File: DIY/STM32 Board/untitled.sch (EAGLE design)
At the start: 13 parts, among them IC2 REG1117, Q1 16 MHz, U1 STM32103RBT6

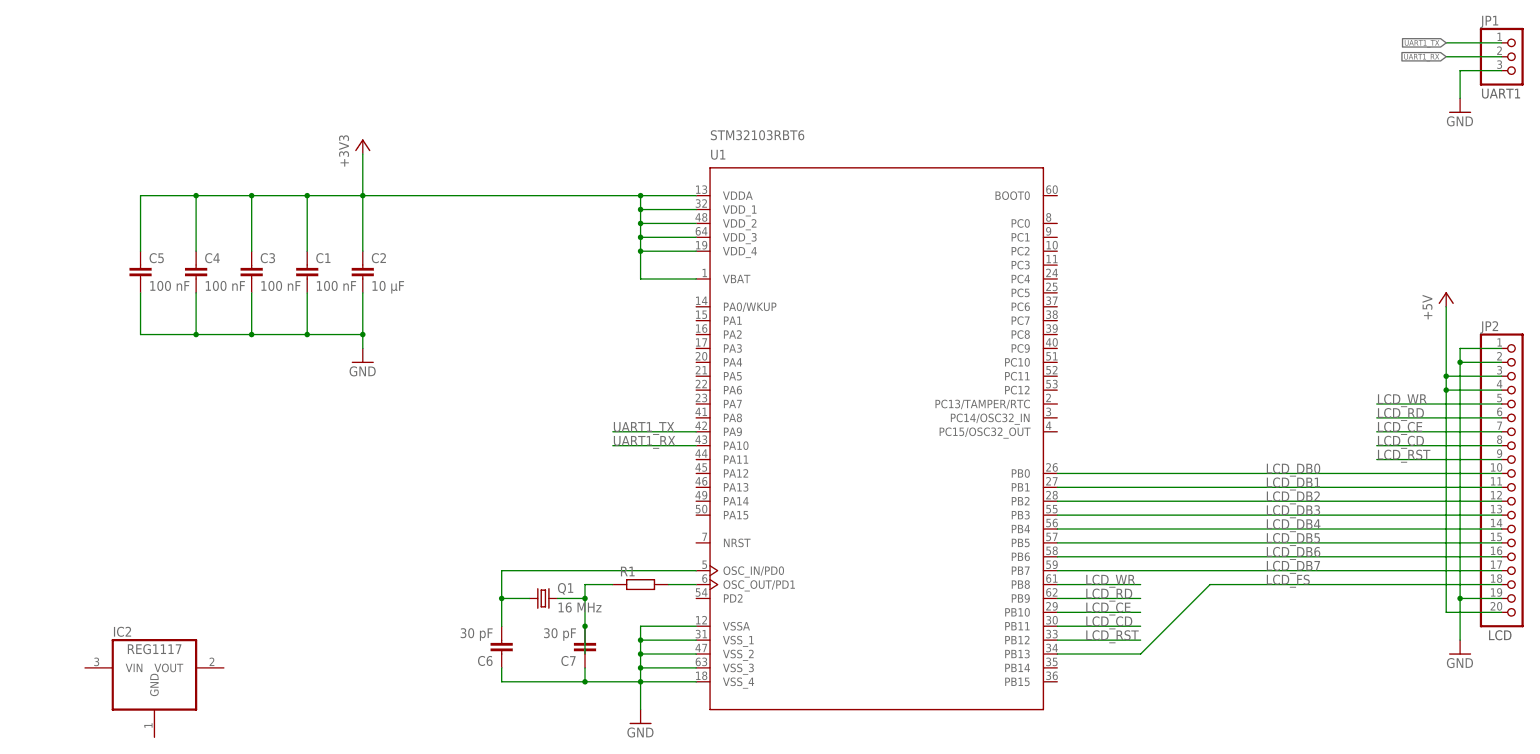
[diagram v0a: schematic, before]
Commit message: DIY ++
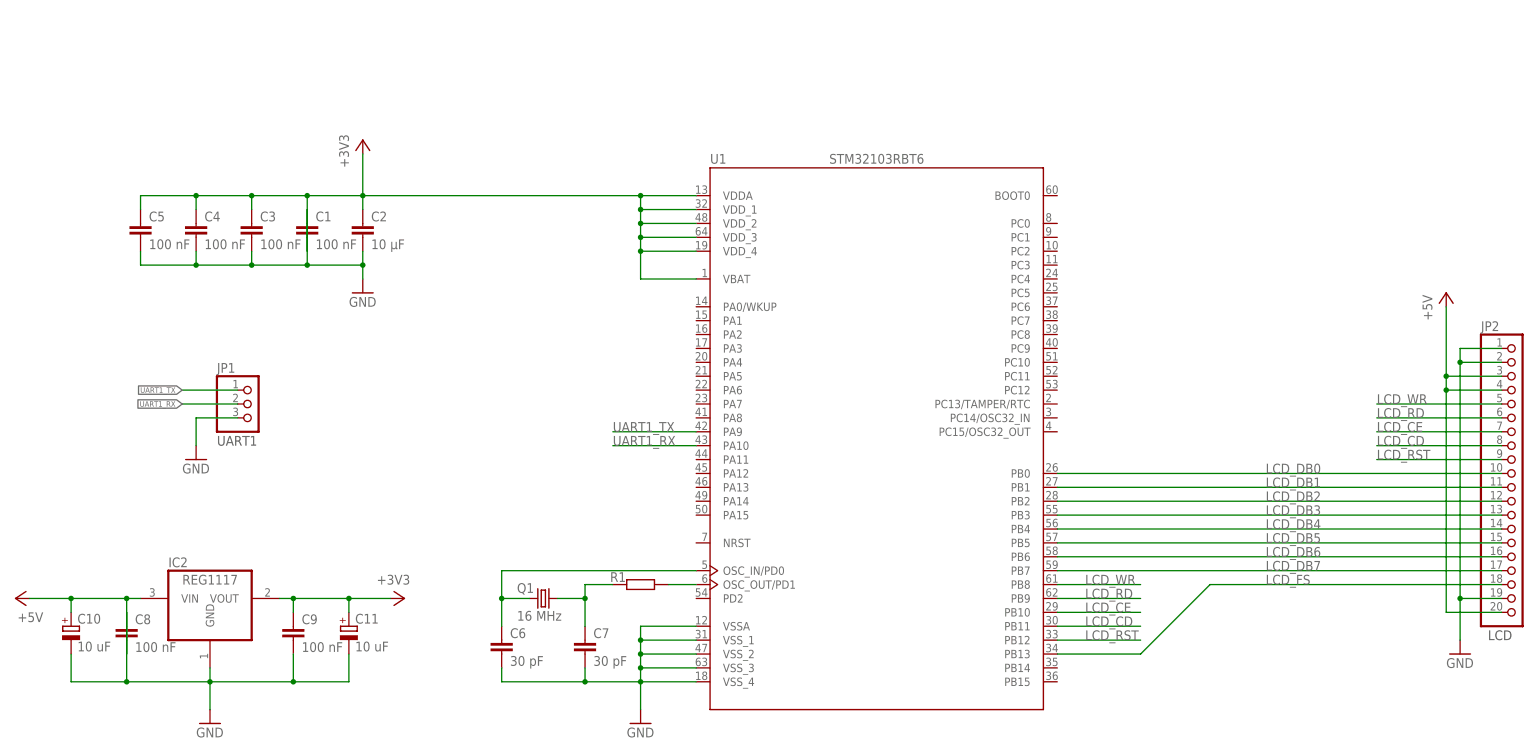
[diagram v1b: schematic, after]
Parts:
- added C10, C11: 10 uF, rcl:CPOL-EUA/3216-18W
- added C8, C9: 100 nF, resistor:C-EUC1206
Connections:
- net +3V3: now also C1.2, C11.+, C9.1, IC2.VOUT; no longer C1.1
- net +5V: now also C10.+, C8.2, IC2.VIN
- net GND: now also C1.1, C10.-, C11.-, C6.2, C7.2, C8.1, C9.2, IC2.GND; no longer C1.2, C6.1, C7.1
- net N$1: now also C6.1; no longer C6.2
- net N$2: now also C7.1; no longer C7.2
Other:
- moved on the sheet: C1, C2, C3, C4, C5, C6, C7, IC2, JP1
